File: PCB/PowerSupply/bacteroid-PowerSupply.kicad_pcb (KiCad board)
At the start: 2 copper layers, 96.5 x 73.7 mm, 15 parts, among them P1 CONN_2, P2 CONN_2, P3 CONN_4, U1 LM7805CT, U2 LM7805CT, U3 LM7809CT, U4 LM7812CT

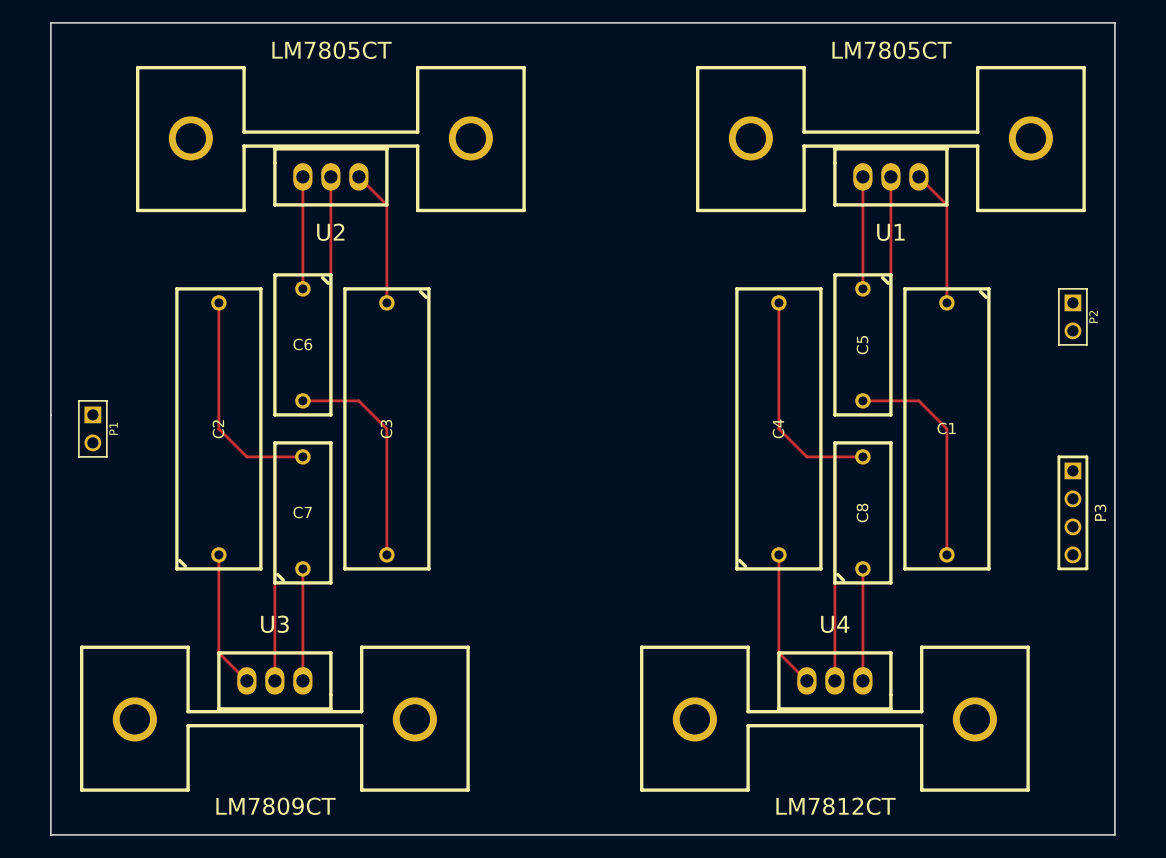
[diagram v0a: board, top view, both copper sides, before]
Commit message: PCB Updates
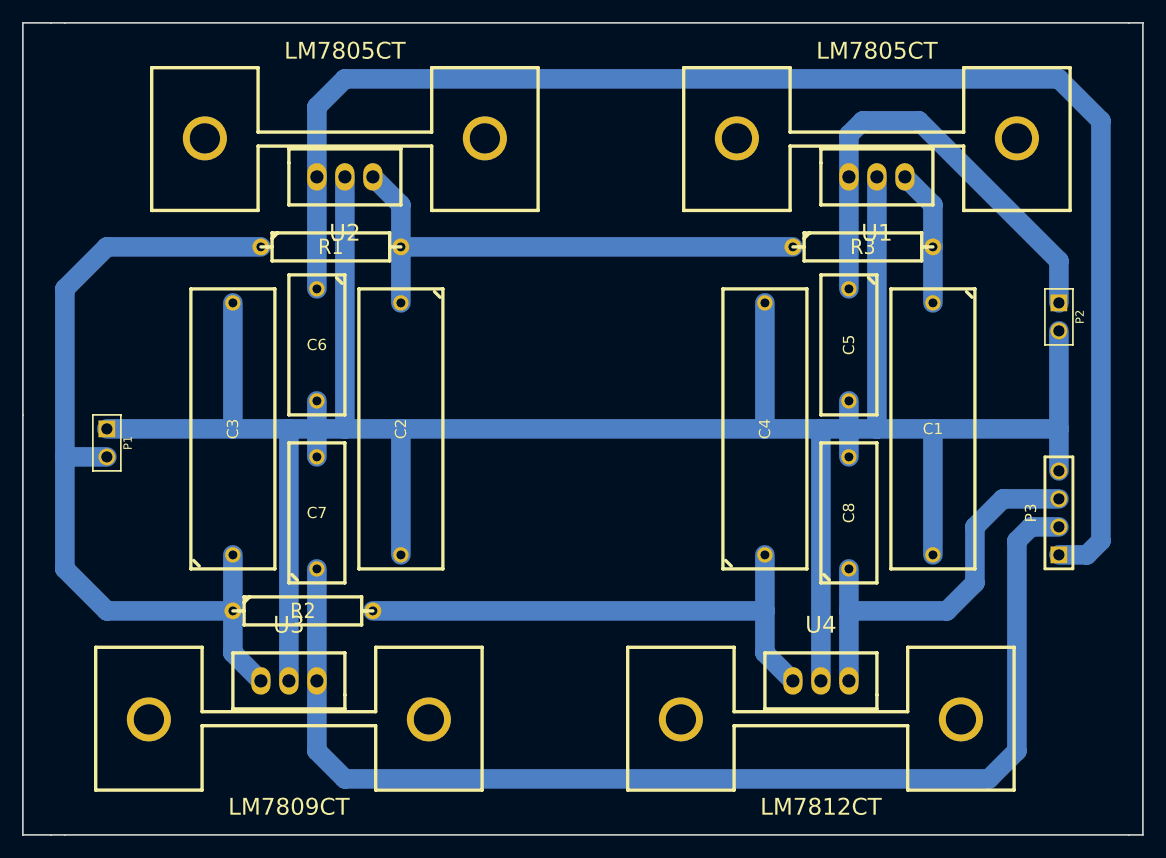
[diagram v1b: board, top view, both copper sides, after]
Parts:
- added R1: 0R, R5, F.Cu at (185.4, 120.7)
- added R2: 0R, R5, F.Cu at (182.9, 153.7)
- added R3: 0R, R5, F.Cu at (233.7, 120.7)
- moved C2 16.5 mm to (191.8, 137.2), turned to 270 degrees
- moved C3 14.0 mm to (176.5, 137.2), turned to 90 degrees
- moved P1 1.80 mm to (165.1, 138.4)
- moved C1 1.27 mm to (240.0, 137.2)
- moved C4 1.27 mm to (224.8, 137.2)
- moved C5 1.27 mm to (232.4, 129.5)
- moved C6 1.27 mm to (184.2, 129.5)
- moved C7 1.27 mm to (184.2, 144.8)
- moved C8 1.27 mm to (232.4, 144.8)
- moved U1 1.27 mm to (234.9, 114.3)
- moved U2 1.27 mm to (186.7, 114.3)
- moved U3 1.27 mm to (181.6, 160.0)
- moved P2 1.27 mm to (251.5, 127.0)
- moved P3 1.27 mm to (251.5, 144.8), turned to 90 degrees
- moved U4 1.27 mm to (229.9, 160.0)
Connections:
- C1 pad 1: +24V -> N-000005
- C2 pad 1: +24V -> N-000003
- C4 pad 1: +24V -> N-000001
- U1 pad 1: +24V -> N-000005
- U2 pad 1: +24V -> N-000003
- U4 pad 1: +24V -> N-000001
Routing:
- net N-000009: track 10.2 -> 132.7 mm
- net N-000002: track 10.2 -> 105.5 mm
- net GND: track 161.7 -> 246.4 mm
- net N-000003: track 0.00 -> 48.0 mm
- net N-000001: track 0.00 -> 48.0 mm
- net N-000004: track 10.2 -> 42.6 mm
- net +24V: track 49.9 -> 77.9 mm
- net N-000008: track 10.2 -> 36.4 mm
- net N-000005: track 0.00 -> 12.5 mm
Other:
- board size 96.5 x 73.7 mm -> 101.6 x 73.7 mm
- net class Default: trace_width 0.254 -> 1.778; via_dia 0.889 -> 1.27
- net class Power added: clearance 0.254, trace_width 1.016, via_dia 0.889, via_drill 0.635
